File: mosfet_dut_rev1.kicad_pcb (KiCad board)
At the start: 2 copper layers, 96.5 x 64.2 mm, 45 parts, among them J1 USB_C_Receptacle_USB2.0_16P, J2 Conn_01x02, J3 Conn_01x02, J4 Conn_01x02, J5 Conn_01x02, J6 Conn_01x02, Q1 AO3400A, Q2 AO3400A, Q3 AO3400A, Q4 AO3400A, SW1 SW_Push, U1 USBLC6-2SC6, U2 ME6211C33M5, U3 CH340C, U4 ESP32-WROOM-32E, U5 74HC4051, U6 INA219AxD

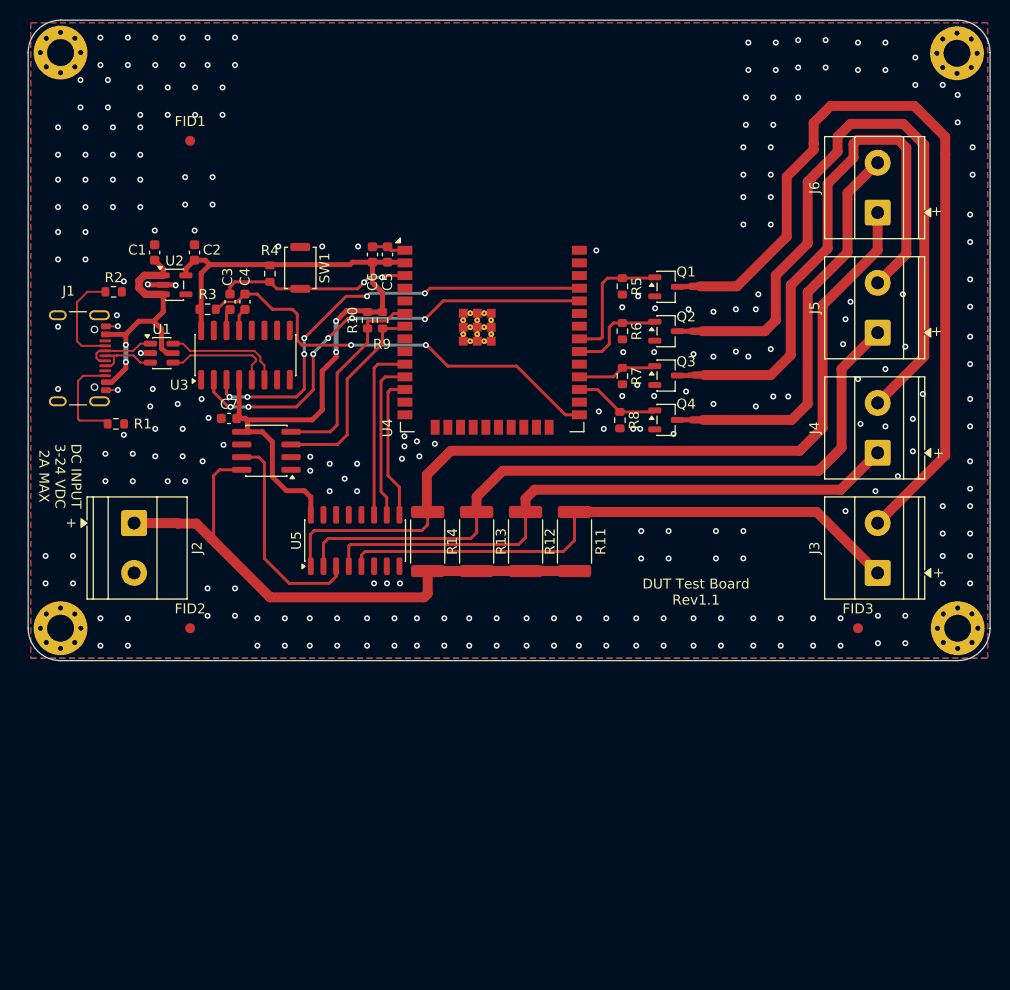
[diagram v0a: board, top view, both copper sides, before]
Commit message: Rev 1.2 Final
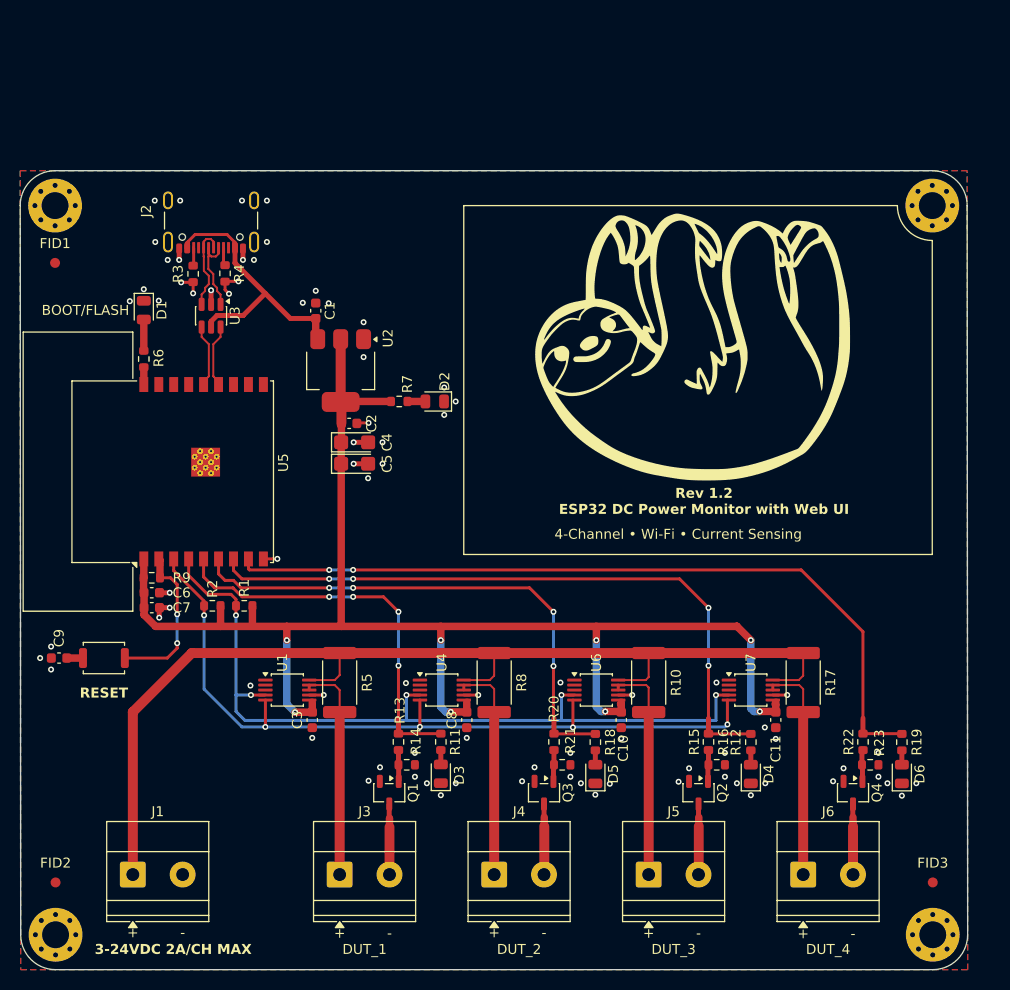
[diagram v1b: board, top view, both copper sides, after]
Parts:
- removed SW1: SW_Push, Button_Switch_SMD:SW_Push_SPST_NO_Alps_SKRK
- added C10: 0.1uF, Capacitor_SMD:C_0603_1608Metric, F.Cu at (154.2, 123.2)
- added C11: 0.1uF, Capacitor_SMD:C_0603_1608Metric, F.Cu at (169.8, 123.2)
- added C8: 0.1uF, Capacitor_SMD:C_0603_1608Metric, F.Cu at (138.8, 123.2)
- added C9: 0.1uF, Capacitor_SMD:C_0603_1608Metric, F.Cu at (97.8, 117.0)
- added D1: LED_R, LED_SMD:LED_0805_2012Metric, F.Cu at (106.3, 82.1)
- added D2: LED_G, LED_SMD:LED_0805_2012Metric, F.Cu at (135.5, 91.2)
- added D3: LED_G, LED_SMD:LED_0805_2012Metric, F.Cu at (136.2, 128.6)
- added D4: LED_G, LED_SMD:LED_0805_2012Metric, F.Cu at (167.2, 128.6)
- added D5: LED_G, LED_SMD:LED_0805_2012Metric, F.Cu at (151.7, 128.6)
- added D6: LED_G, LED_SMD:LED_0805_2012Metric, F.Cu at (182.4, 128.6)
- added R15: 5k1, Resistor_SMD:R_0603_1608Metric, F.Cu at (163.0, 125.4)
- added R16: 100k, Resistor_SMD:R_0603_1608Metric, F.Cu at (163.8, 127.7)
- added R17: 2m, Resistor_SMD:R_2512_6332Metric, F.Cu at (172.5, 119.5)
- added R18: 1k, Resistor_SMD:R_0603_1608Metric, F.Cu at (151.7, 125.4)
- added R19: 1k, Resistor_SMD:R_0603_1608Metric, F.Cu at (182.4, 125.4)
- added R20: 5k1, Resistor_SMD:R_0603_1608Metric, F.Cu at (147.5, 125.4)
- added R21: 100k, Resistor_SMD:R_0603_1608Metric, F.Cu at (148.3, 127.7)
- added R22: 5k1, Resistor_SMD:R_0603_1608Metric, F.Cu at (178.5, 125.4)
- added R23: 100k, Resistor_SMD:R_0603_1608Metric, F.Cu at (179.2, 127.7)
- added RESET: SW_Push, Button_Switch_SMD:SW_Push_SPST_NO_Alps_SKRK, F.Cu at (102.3, 117.0)
- added U7: INA226, Package_SO:VSSOP-10_3x3mm_P0.5mm, F.Cu at (167.2, 120.2)
- C2: value 1uF -> 0.1uF
- C4, C5: value 0.1uF -> 10uF; footprint Capacitor_SMD:C_0603_1608Metric -> Capacitor_Tantalum_SMD:CP_EIA-3216-18_Kemet-A
- C6: value 10uF -> 0.1uF
- C7: value 0.1uF -> 1uF
- J1: value USB_C_Receptacle_USB2.0_16P -> SCREW_TERMINAL; footprint Connector_USB:USB_C_Receptacle_GCT_USB4105-xx-A_16P_TopMnt_Horizontal -> TerminalBlock_Phoenix:TerminalBlock_Phoenix_MKDS-1,5-2_1x02_P5.00mm_Horizontal
- J2: value Conn_01x02 -> USB_C_Receptacle_USB2.0_16P; footprint TerminalBlock_Phoenix:TerminalBlock_Phoenix_MKDS-1,5-2_1x02_P5.00mm_Horizontal -> Connector_USB:USB_C_Receptacle_GCT_USB4105-xx-A_16P_TopMnt_Horizontal
- J3, J4, J5, J6: value Conn_01x02 -> SCREW_TERMINAL
- R10, R5, R8: value 5k1 -> 2m; footprint Resistor_SMD:R_0603_1608Metric -> Resistor_SMD:R_2512_6332Metric
- R11, R12: value 50m -> 1k; footprint Resistor_SMD:R_2512_6332Metric -> Resistor_SMD:R_0603_1608Metric
- R13: value 50m -> 5k1; footprint Resistor_SMD:R_2512_6332Metric -> Resistor_SMD:R_0603_1608Metric
- R14: value 50m -> 100k; footprint Resistor_SMD:R_2512_6332Metric -> Resistor_SMD:R_0603_1608Metric
- R6, R7: value 5k1 -> 1k
- U1: value USBLC6-2SC6 -> INA226; footprint Package_TO_SOT_SMD:SOT-23-6 -> Package_SO:VSSOP-10_3x3mm_P0.5mm
- U2: value ME6211C33M5 -> AMS1117-3.3; footprint Package_TO_SOT_SMD:SOT-23-5 -> Package_TO_SOT_SMD:SOT-223-3_TabPin2
- U3: value CH340C -> USBLC6-2SC6; footprint Package_SO:SOIC-16_3.9x9.9mm_P1.27mm -> Package_TO_SOT_SMD:SOT-23-6
- U4: value ESP32-WROOM-32E -> INA226; footprint RF_Module:ESP32-WROOM-32E -> Package_SO:VSSOP-10_3x3mm_P0.5mm
- U5: value 74HC4051 -> ESP32-C3-WROOM-02; footprint Package_SO:SO-16_3.9x9.9mm_P1.27mm -> RF_Module:ESP32-C3-WROOM-02
- U6: value INA219AxD -> INA226; footprint Package_SO:SOIC-8_3.9x4.9mm_P1.27mm -> Package_SO:VSSOP-10_3x3mm_P0.5mm
- moved H4 92.7 mm to (185.5, 144.8), turned to -90 degrees
- moved H2 91.8 mm to (97.5, 71.6), turned to -90 degrees
- moved H1 88.5 mm to (97.5, 144.8), turned to -90 degrees
- moved J6 66.8 mm to (172.5, 138.7), turned to 0 degrees
- moved J3 61.9 mm to (126.0, 138.7), turned to 0 degrees
- moved J5 59.0 mm to (157.0, 138.7), turned to 0 degrees
- moved Q1 57.9 mm to (131.0, 130.5), turned to -90 degrees
- moved J4 57.2 mm to (141.5, 138.7), turned to 0 degrees
- moved J1 52.2 mm to (105.2, 138.7), turned to 0 degrees
- moved R5 48.8 mm to (126.0, 119.5), turned to 90 degrees
- moved R6 48.1 mm to (106.3, 87.0), turned to 90 degrees
- moved Q2 46.4 mm to (162.0, 130.5), turned to -90 degrees
- moved R10 46.0 mm to (157.0, 119.5), turned to 90 degrees
- moved Q3 43.6 mm to (146.5, 130.5), turned to -90 degrees
- moved C3 42.8 mm to (123.2, 123.2), turned to -90 degrees
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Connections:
- net /OUT1- renamed /DUT1-
- net /OUT4- renamed /DUT4-
- C3 pad 1: /UARTDDTR -> +3V3
- C3 pad 2: /UARTDDTR_EN -> GND
- C4 pad 1: /UARTDRTS_IO0 -> +3V3
- C4 pad 2: /UARTDRTS -> GND
- C5 pad 1: GND -> +3V3
- C5 pad 2: +3V3 -> GND
- C6 pad 1: GND -> +3V3
- C6 pad 2: +3V3 -> GND
- C7 pad 1: GND -> +3V3
- C7 pad 2: +3V3 -> GND
- J3 pad 1: /OUT1+ -> /DUT1+
- J4 pad 1: /OUT2+ -> /DUT2+
- J4 pad 2: /OUT2- -> /DUT2-
- J5 pad 1: /OUT3+ -> /DUT3+
- J5 pad 2: /OUT3- -> /DUT3-
- J6 pad 1: /OUT4+ -> /DUT4+
- Q1 pad 1: /M1_CTRL -> Net-(Q1-G)
- Q2 pad 1: /M2_CTRL -> Net-(Q2-G)
- Q2 pad 3: /OUT2- -> /DUT3-
- Q3 pad 1: /M3_CTRL -> Net-(Q3-G)
- Q3 pad 3: /OUT3- -> /DUT2-
- Q4 pad 1: /M4_CTRL -> Net-(Q4-G)
- R1 pad 1: /USBCC2 -> +3V3
- R1 pad 2: GND -> /I2C_SDA
- R10 pad 1: +3V3 -> /DUT3+
- R10 pad 2: /I2C_SCL -> /POWER_SENSE+
- R11 pad 1: /OUT1+ -> /M1_CTRL
- R11 pad 2: /POWER_SENSE+ -> Net-(D3-A)
- R12 pad 1: /OUT2+ -> /M3_CTRL
- R12 pad 2: /POWER_SENSE+ -> Net-(D4-A)
- R13 pad 1: /OUT3+ -> Net-(Q1-G)
- R13 pad 2: /POWER_SENSE+ -> /M1_CTRL
- R14 pad 1: /OUT4+ -> Net-(Q1-G)
- R14 pad 2: /POWER_SENSE+ -> GND
- R2 pad 1: /USBCC1 -> +3V3
- R2 pad 2: GND -> /I2C_SCL
- R3 pad 1: +3V3 -> /USBCC2
- R3 pad 2: /UARTDRTS_IO0 -> GND
- R4 pad 1: +3V3 -> /USBCC1
- R4 pad 2: /UARTDDTR_EN -> GND
- R5 pad 1: /M1_CTRL -> /DUT1+
- R5 pad 2: GND -> /POWER_SENSE+
- R6 pad 1: /M2_CTRL -> Net-(U5-IO0)
- R6 pad 2: GND -> Net-(D1-A)
- R7 pad 1: /M3_CTRL -> +3V3
- R7 pad 2: GND -> Net-(D2-A)
- R8 pad 1: /M4_CTRL -> /DUT2+
- R8 pad 2: GND -> /POWER_SENSE+
- R9 pad 2: /I2C_SDA -> /ENABLE
- U1 pad 1: /USBCD- -> GND
- U1 pad 3: /USBCD+ -> unconnected-(U1-~{Alert}-Pad3)
- U1 pad 4: /USBD+ -> /I2C_SDA
- U1 pad 5: +VBUS -> /I2C_SCL
- U1 pad 6: /USBD- -> +3V3
- U2 pad 1: +VBUS -> GND
- U2 pad 2: GND -> +3V3
- U3 pad 1: GND -> /USBCD-
- U3 pad 2: /UARTDRX -> GND
- U3 pad 3: /UARTDTX -> /USBCD+
- U3 pad 4: +3V3 -> /USBC_DP
- U3 pad 5: /USBD+ -> +VBUS
- U3 pad 6: /USBD- -> /USBC_DN
- U4 pad 10: /GPIO25 -> /POWER_SENSE+
- U4 pad 2: +3V3 -> GND
- U4 pad 3: /UARTDDTR_EN -> unconnected-(U4-~{Alert}-Pad3)
- U4 pad 4: unconnected-(U4-SENSOR_VP-Pad4) -> /I2C_SDA
- U4 pad 5: unconnected-(U4-SENSOR_VN-Pad5) -> /I2C_SCL
- U4 pad 6: /I2C_SCL -> +3V3
- U4 pad 7: /I2C_SDA -> GND
- U4 pad 8: unconnected-(U4-IO32-Pad8) -> /DUT2+
- U4 pad 9: unconnected-(U4-IO33-Pad9) -> /DUT2+
- U5 pad 1: /OUT4+ -> +3V3
- U5 pad 10: /GPIO26 -> unconnected-(U5-IO10-Pad10)
- U5 pad 11: /GPIO25 -> unconnected-(U5-IO20/RXD-Pad11)
- U5 pad 13: unconnected-(U5-A0-Pad13) -> /USBC_DN
- U5 pad 14: unconnected-(U5-A1-Pad14) -> /USBC_DP
- U5 pad 16: +3V3 -> unconnected-(U5-IO2-Pad16)
- U5 pad 2: /OUT3+ -> /ENABLE
- U5 pad 3: /IN- -> /I2C_SCL
- U5 pad 4: /OUT2+ -> /I2C_SDA
- U5 pad 5: /OUT1+ -> /M1_CTRL
- U5 pad 6: GND -> /M2_CTRL
- U5 pad 7: GND -> /M3_CTRL
- U5 pad 8: GND -> /M4_CTRL
- U5 pad 9: /GPIO27 -> GND
- U6 pad 3: /I2C_SDA -> unconnected-(U6-~{Alert}-Pad3)
- U6 pad 4: /I2C_SCL -> /I2C_SDA
- U6 pad 5: +3V3 -> /I2C_SCL
- U6 pad 6: GND -> +3V3
- U6 pad 7: /IN- -> GND
- U6 pad 8: /POWER_SENSE+ -> /DUT3+
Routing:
- net /OUT4+: track 86.0 -> 0.00 mm
- net /DUT1-: track 82.3 -> 7.08 mm
- net /OUT3+: track 73.4 -> 0.00 mm
- net +3V3: track 78.2 -> 151.1 mm, vias 2 -> 8
- net /M4_CTRL: track 8.56 -> 79.4 mm, vias 0 -> 2
- net /OUT2-: track 69.2 -> 0.00 mm
- net /OUT2+: track 61.2 -> 0.00 mm
- net /I2C_SDA: track 20.5 -> 81.7 mm, vias 0 -> 5
- net /M3_CTRL: track 8.01 -> 67.2 mm, vias 0 -> 4
- net /OUT1+: track 58.9 -> 0.00 mm
- net /I2C_SCL: track 20.6 -> 79.2 mm, vias 0 -> 5
- net /OUT3-: track 56.6 -> 0.00 mm
- net /POWER_SENSE+: track 59.2 -> 108.1 mm
- net /UARTDRX: track 45.2 -> 0.00 mm, vias 6 -> 0
- net /UARTDTX: track 44.5 -> 0.00 mm, vias 6 -> 0
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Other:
- board size 96.5 x 64.2 mm -> 95 x 80.2 mm
- board text added: "-"
- board text added: "3-24VDC 2A/CH MAX"
- board text added: "4-Channel • Wi-Fi • Current Sensing"
- board text added: "BOOT/FLASH"
- board text added: "DUT_1"
- board text added: "DUT_2"
- board text added: "DUT_3"
- board text added: "DUT_4"
- board text added: "Rev 1.2 ESP32 DC Power Monitor with Web UI"
- board text removed: "DC INPUT 3-24 VDC 2A MAX"
- board text removed: "DUT Test Board Rev1.1"
